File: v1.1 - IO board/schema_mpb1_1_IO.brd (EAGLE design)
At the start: 178.4 x 50.8 mm, 82 parts

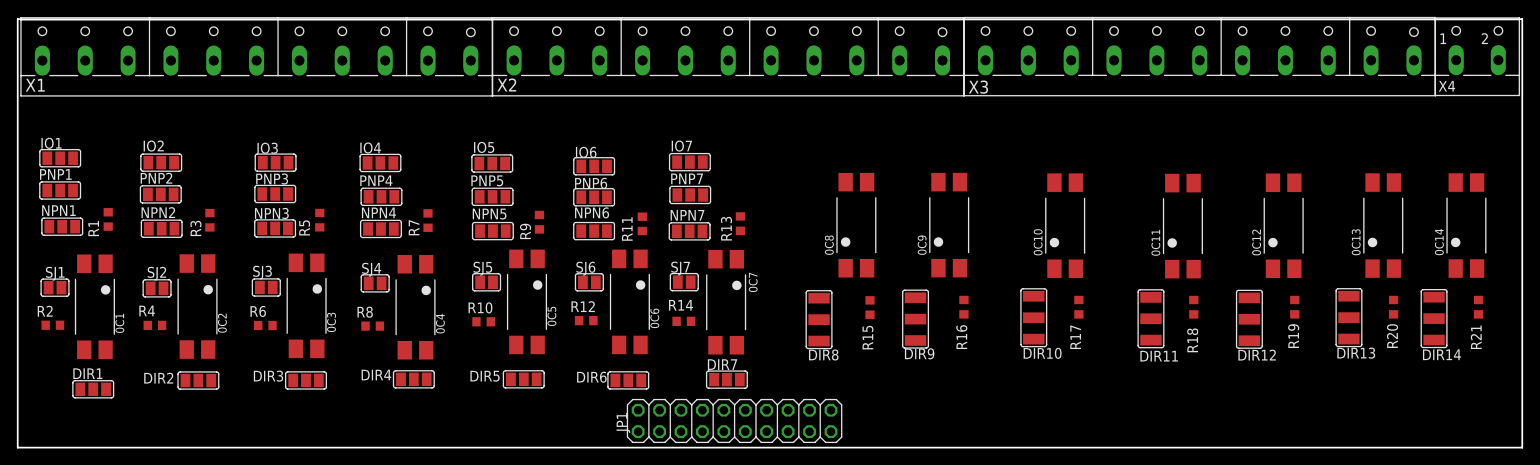
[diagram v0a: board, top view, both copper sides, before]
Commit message: First Revision
- Added 3 PIN terminal block for power
- Cleaned up tracks /rerouted
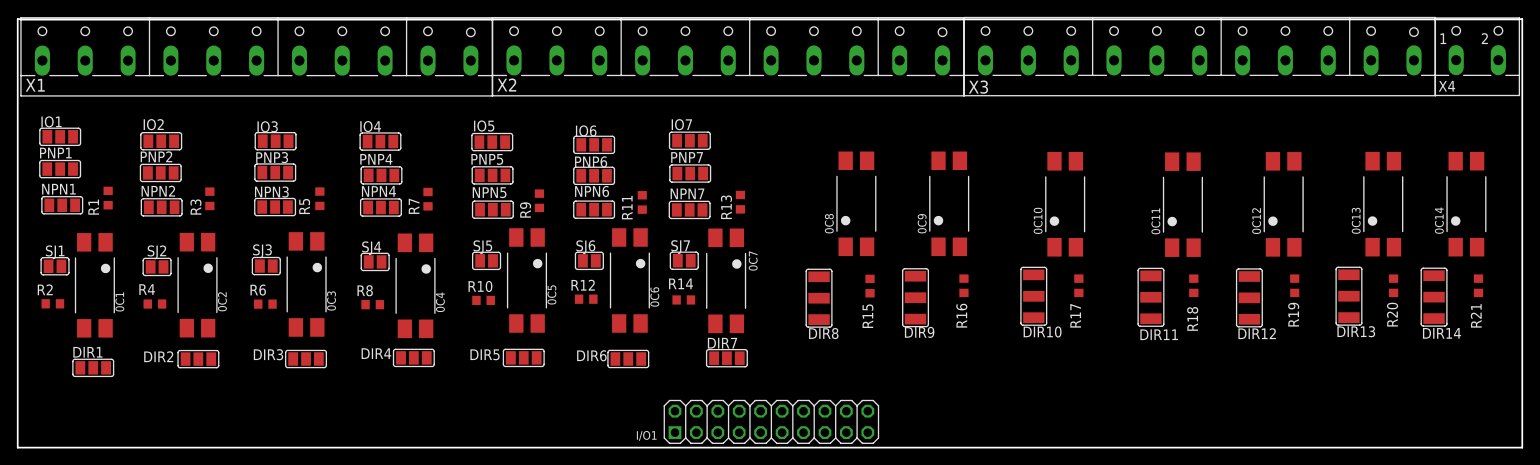
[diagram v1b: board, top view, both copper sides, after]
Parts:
- removed JP1: (no value), pinhead:2X10
- added I/O1: (no value), pinhead-2:2X10
- moved 0C10 2.54 mm to (124.2, 23.5)
- moved 0C11 2.54 mm to (138.2, 23.5)
- moved 0C13 2.54 mm to (162.0, 23.5)
- moved 0C14 2.54 mm to (171.8, 23.5)
- moved 0C9 2.54 mm to (110.5, 23.6)
- moved IO1 2.54 mm to (5.08, 31.5)
- moved IO5 2.54 mm to (56.3, 30.9)
- moved NPN2 2.54 mm to (17.1, 23.2)
- moved NPN5 2.54 mm to (56.4, 22.9)
- moved NPN6 2.54 mm to (68.4, 22.9)
- moved PNP4 2.54 mm to (43.2, 26.9)
- moved PNP5 2.54 mm to (56.3, 26.9)
- moved 0C2 2.54 mm to (21.4, 13.9)
- moved 0C4 2.54 mm to (47.2, 13.8)
- moved 0C5 2.54 mm to (60.4, 14.5)
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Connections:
- new net +12V: I/O1.20
- new net +5V: I/O1.19
- new net 3.3V: I/O1.17
- new net VIN: I/O1.18
- net GND: now also I/O1.15, I/O1.16
- net PE0: now also I/O1.1
- net PE1: now also I/O1.2
- net PE10: now also I/O1.11
- net PE11: now also I/O1.12
- net PE12: now also I/O1.13
- net PE13: now also I/O1.14
- net PE2: now also I/O1.3
- net PE3: now also I/O1.4
- net PE4: now also I/O1.5
- net PE5: now also I/O1.6
- net PE6: now also I/O1.7
- net PE7: now also I/O1.8
- net PE8: now also I/O1.9
- net PE9: now also I/O1.10
